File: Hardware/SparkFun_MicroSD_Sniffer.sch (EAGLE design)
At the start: 9 parts, among them U1 MICRO-SDCARD, U2 microSD Socket

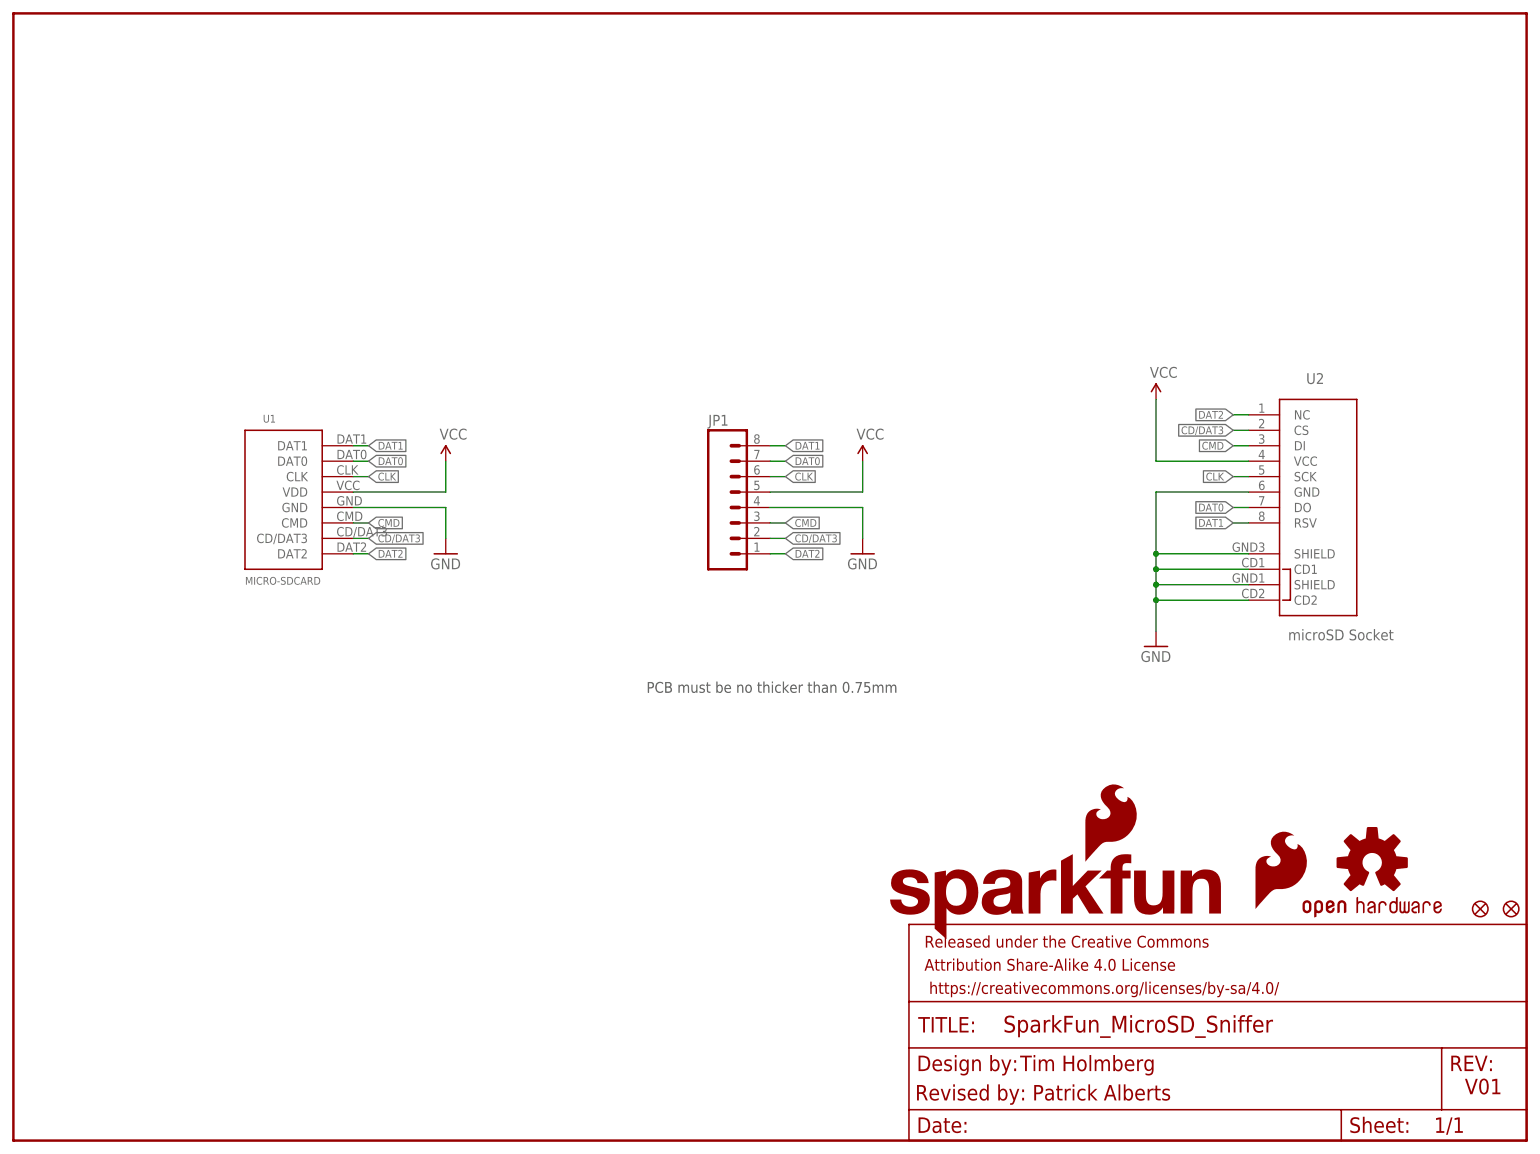
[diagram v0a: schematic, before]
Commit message: changed schematic and board design
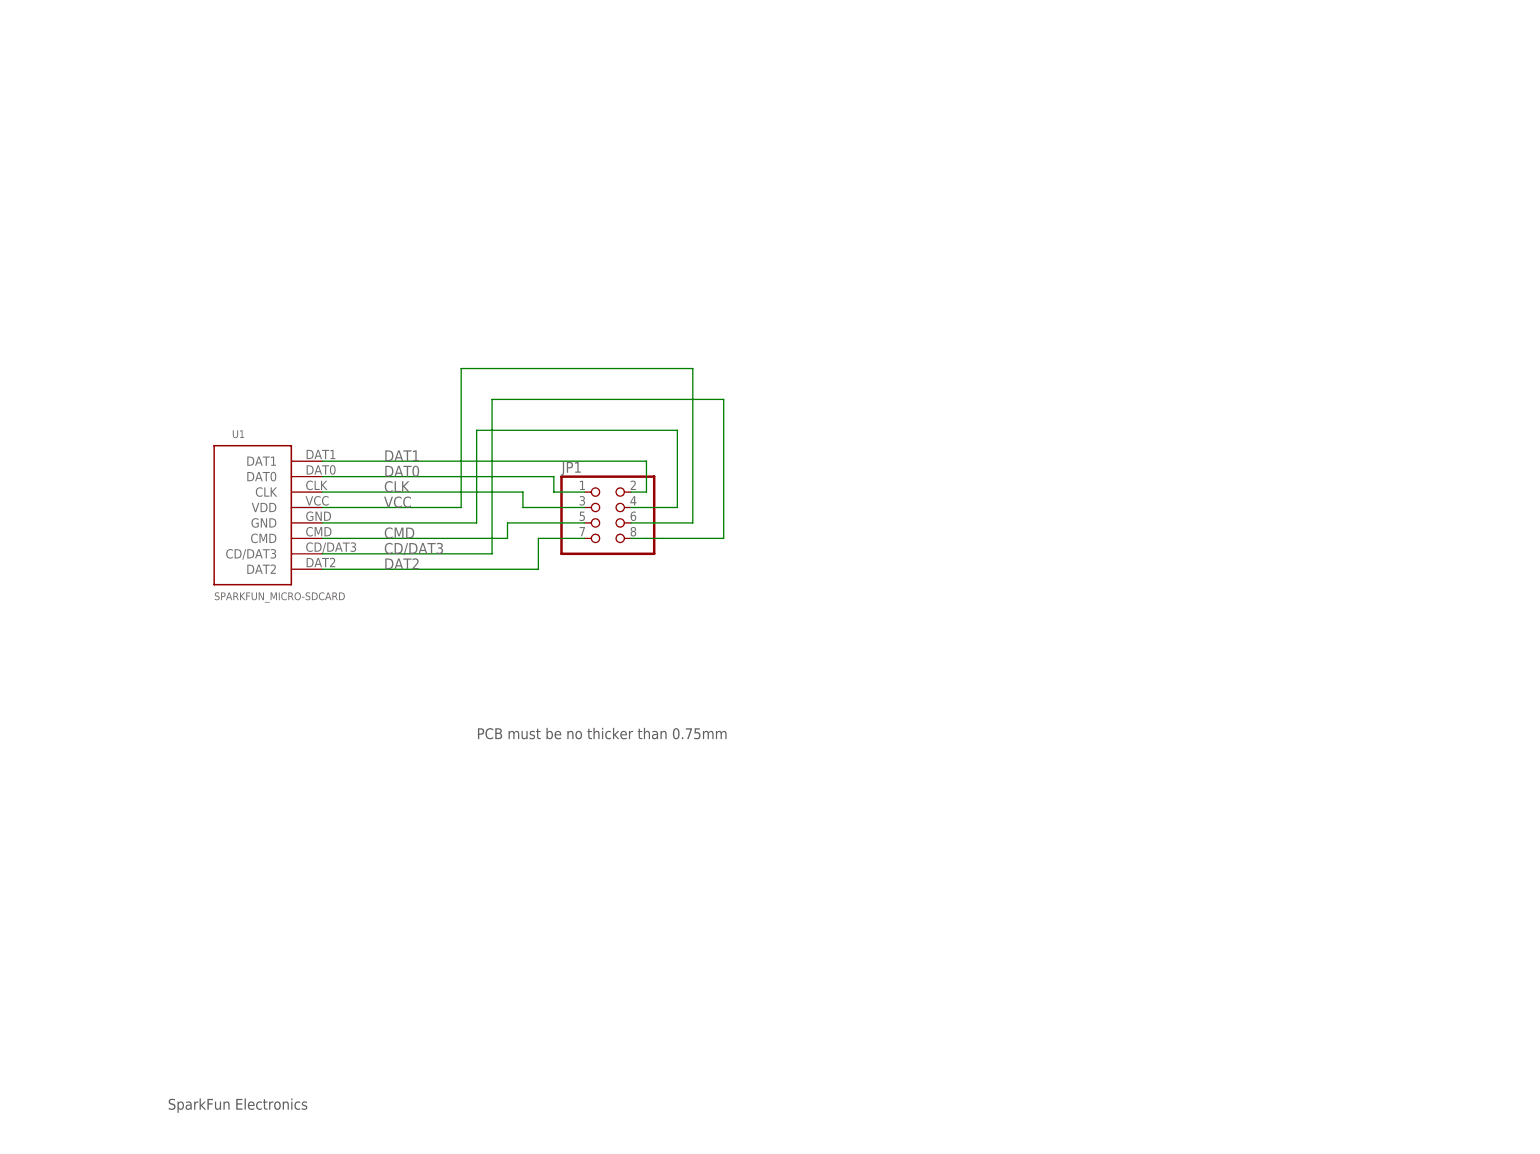
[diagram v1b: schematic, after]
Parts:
- removed FID1, FID2: FIDUCIAL1X2, SparkFun-Aesthetics:FIDUCIAL1X2
- removed FRAME1: (no value), SparkFun-Aesthetics:FRAME-LETTER
- removed LOGO1: OSHW-LOGOM, SparkFun-Aesthetics:OSHW-LOGOM
- removed LOGO2: SFE_LOGO_FLAME.2_INCH, SparkFun-Aesthetics:SFE_LOGO_FLAME.2_INCH
- removed LOGO3: SFE_LOGO_NAME_FLAME.1_INCH, SparkFun-Aesthetics:SFE_LOGO_NAME_FLAME.1_INCH
- removed U2: microSD Socket, SparkFun-Connectors:USD-SOCKET
- JP1: device SparkFun:M08 -> pinhead:PINHD-2X4
- U1: value MICRO-SDCARD -> SPARKFUN_MICRO-SDCARD; device SparkFun-Boards:MICRO-SDCARD -> microsniffer-v14:SPARKFUN_MICRO-SDCARD
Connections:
- net CD/DAT3: now also JP1.8; no longer JP1.2, U2.CS
- net CLK: now also JP1.3; no longer JP1.6, U2.SCK
- net CMD: now also JP1.5; no longer JP1.3, U2.DI
- net DAT0: now also JP1.1; no longer JP1.7, U2.DO
- net DAT1: now also JP1.2; no longer JP1.8, U2.RSV
- net DAT2: now also JP1.7; no longer JP1.1, U2.NC
- net GND: no longer U2.CD1, U2.CD2, U2.GND, U2.SHIELD@1, U2.SHIELD@3
- net VCC: now also JP1.6; no longer JP1.5, U2.VCC
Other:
- note added: "SparkFun Electronics"
- note removed: "Revised by: Patrick Alberts"
- note removed: "Tim Holmberg"
- note removed: "V01"
- moved on the sheet: U1
